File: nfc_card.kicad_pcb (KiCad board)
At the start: 2 copper layers, 2 parts, among them U1 ST25DV04K-JFR6D3

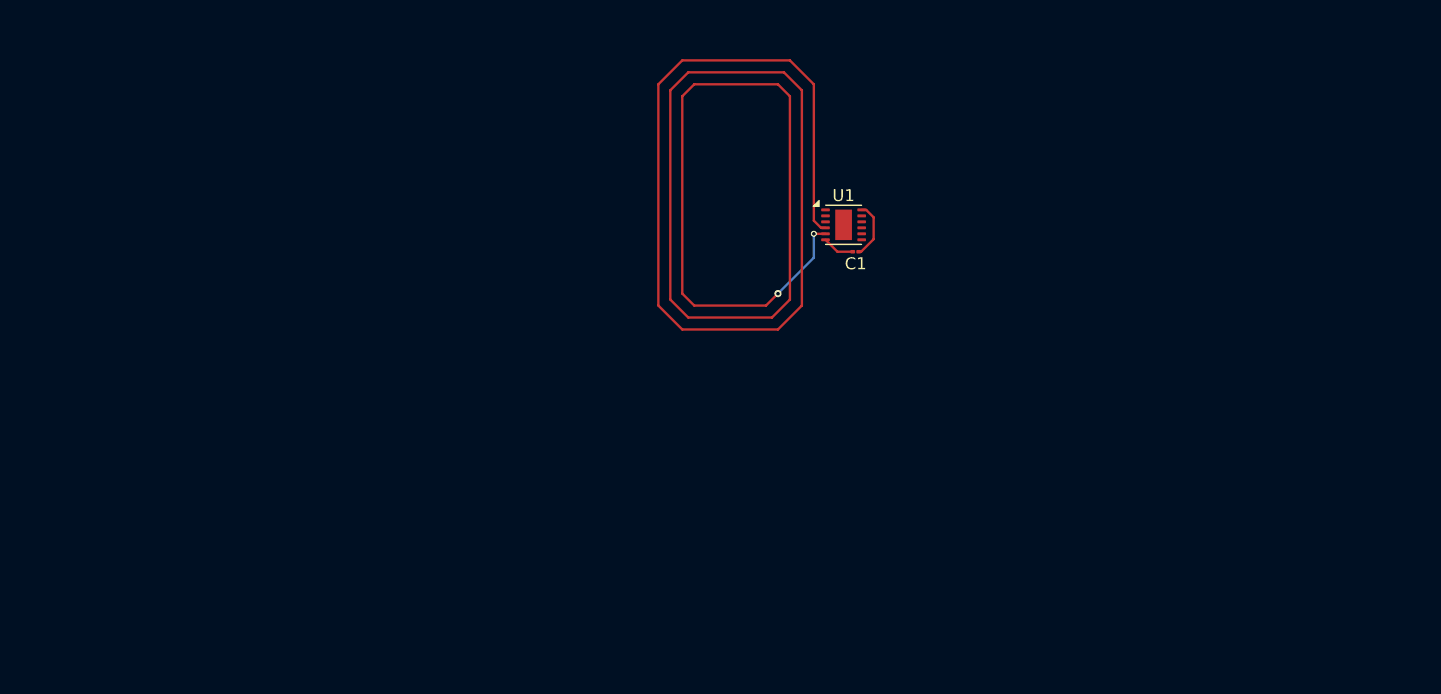
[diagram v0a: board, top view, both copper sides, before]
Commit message: stufffff
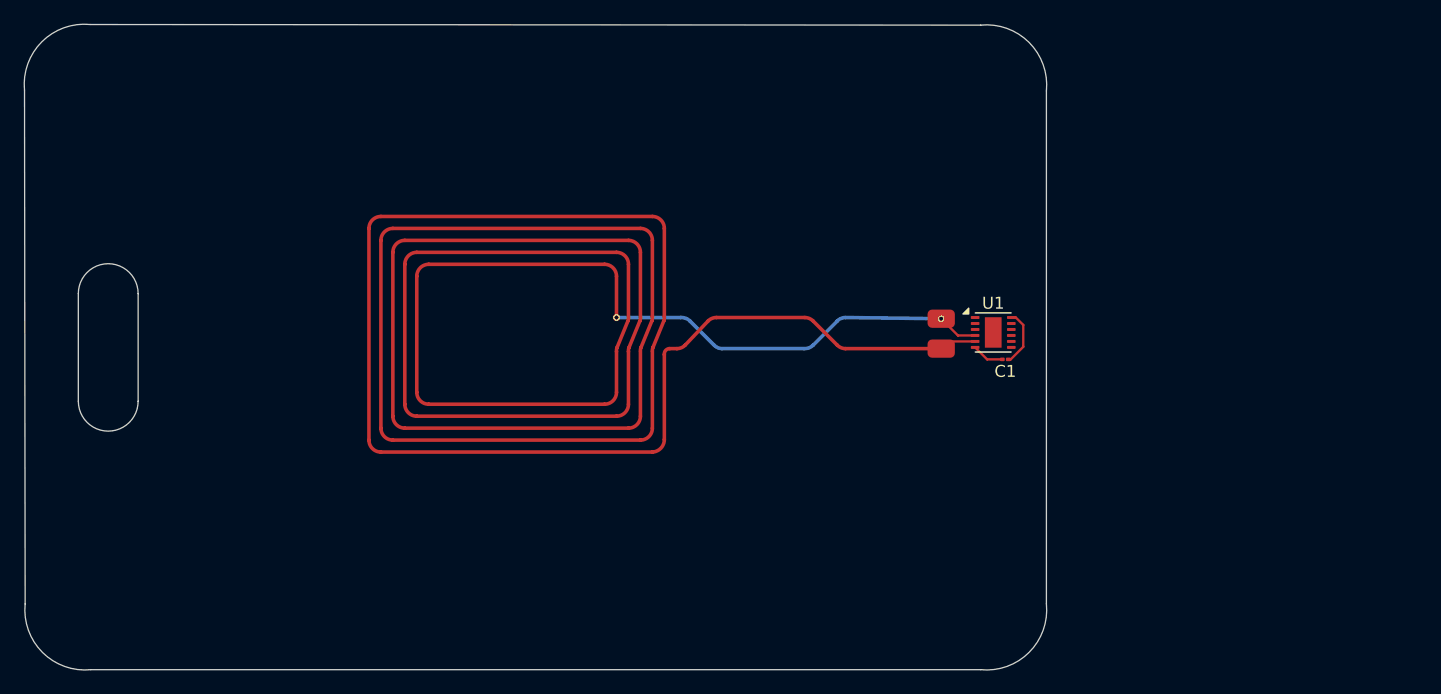
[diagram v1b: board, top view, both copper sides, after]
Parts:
- added U2: NFC_ANTENNA, Library:NFC_ANT, F.Cu at (154.7, 104.1)
- moved C1 15.4 mm to (152.0, 105.0)
- moved U1 15.4 mm to (151.0, 102.8)
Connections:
- U1 pad 5: Net-(U1-AC0) -> Net-(U1-AC1)
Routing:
- net Net-(U1-AC0): track 177.8 -> 2.82 mm, vias 2 -> 0
- net Net-(U1-AC1): track 0.00 -> 2.64 mm
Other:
- board outline added: 85.5 x 54 mm

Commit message: bit of design, needs to be finished
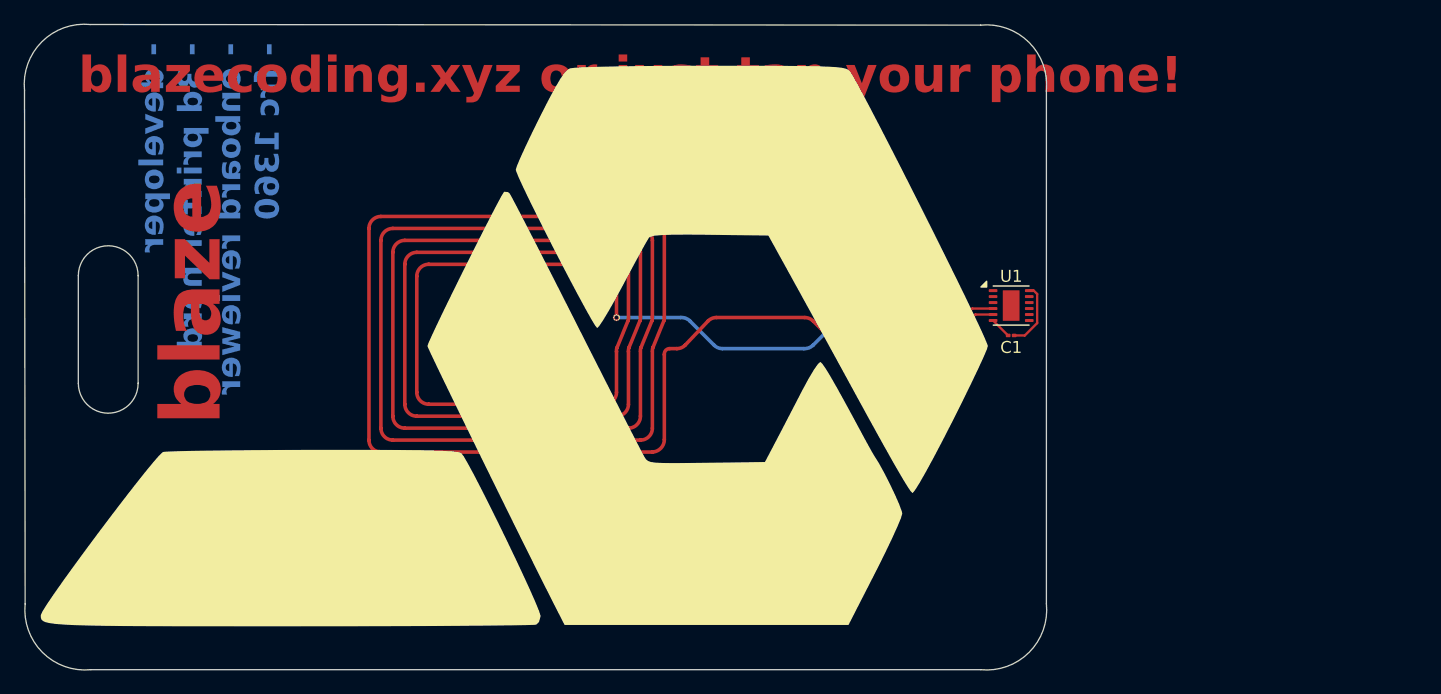
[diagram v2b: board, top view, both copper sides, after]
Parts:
- added G***: LOGO, LOGO, F.Cu at (112.0, 104.0)
- moved U1 2.70 mm to (152.5, 100.5)
- moved C1 2.06 mm to (152.5, 103.0)
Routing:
- net Net-(U1-AC1): track 2.64 -> 5.07 mm
- net Net-(U1-AC0): track 2.82 -> 4.44 mm
- net Net-(U1-VSS): track 2.69 -> 1.78 mm
- net Net-(U1-VCC): track 4.77 -> 5.56 mm
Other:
- outline, holes or cut-outs redrawn
- board text added: "- developer - 3d printer nerd - onboard reviewer - frc 1360"
- board text added: "blaze"
- board text added: "blazecoding.xyz or just tap your phone!"
